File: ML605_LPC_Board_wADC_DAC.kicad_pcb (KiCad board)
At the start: 4 copper layers, 100.1 x 99.7 mm, 122 parts, among them IC1 ADC10D040CIVS_NOPB, IC2 AD8137YRZ-REEL, IC3 AD8137YRZ-REEL, IC4 DAC5652IPFB, J1 ASP-134604-01, J10 Conn_02x06_Odd_Even, J11 Conn_02x06_Odd_Even, J12 Conn_02x06_Odd_Even, J13 Conn_01x03_Pin, J14 Conn_01x03_Pin, J2 Conn_01x03_Pin, J3 Conn_01x03_Pin, J4 SMA Connector, J5 SMA Connector, J6 Conn_01x03_Pin, J7 Conn_01x03_Pin, J8 SMA Connector, J9 SMA Connector, U1 LMV7219M7, U2 LMV7219M7, U3 NCV317, U4 LMH6720MA, U5 LMH6720MA

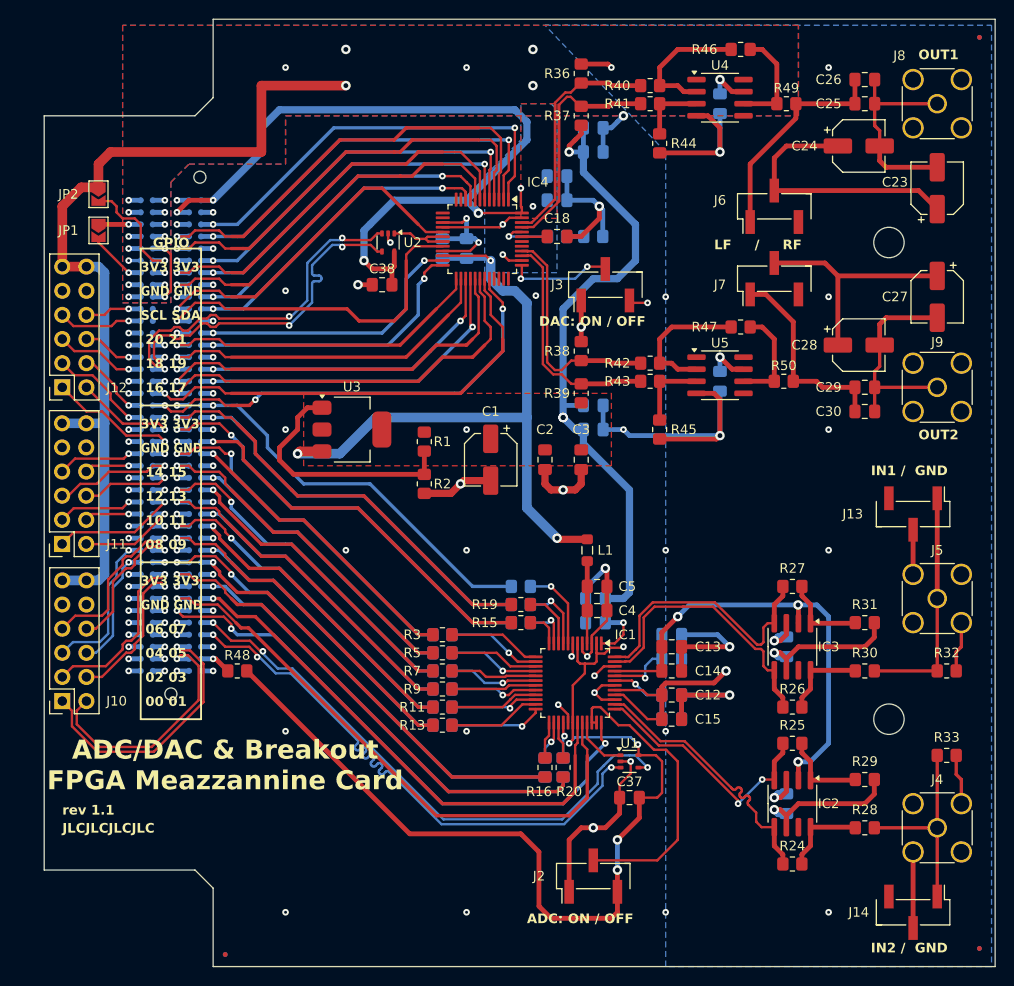
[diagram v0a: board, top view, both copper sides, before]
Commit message: Fixed pcb dimensions (again)
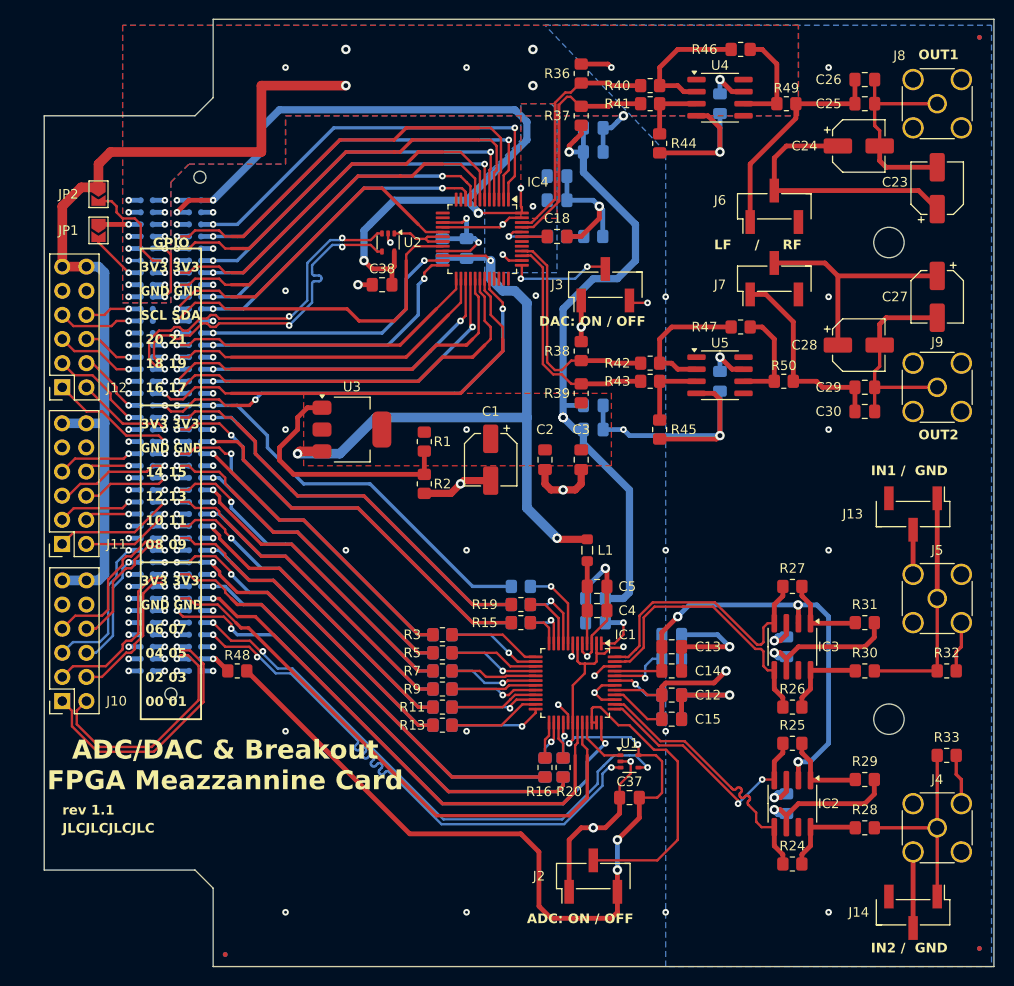
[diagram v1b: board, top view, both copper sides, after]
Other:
- board size 100.1 x 99.7 mm -> 99.9 x 99.7 mm
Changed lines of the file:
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@@
 		(pts
 			(xy 90.875 139.205) (xy 75 139.205) (xy 75 59.83) (xy 90.875 59.83) (xy 92.78 57.925) (xy 92.78 49.67)
-			(xy 175.076 49.67) (xy 175.076 149.365) (xy 92.78 149.365) (xy 92.78 141.11)
+			(xy 174.949 49.67) (xy 174.949 149.365) (xy 92.78 149.365) (xy 92.78 141.11)
 		)
 		(stroke
@@
 		(polygon
 			(pts
-				(xy 75 49.67) (xy 175.076 49.67) (xy 175.076 149.365) (xy 75 149.365)
+				(xy 75 49.67) (xy 174.949 49.67) (xy 174.949 149.365) (xy 75 149.365)
 			)
 		)
